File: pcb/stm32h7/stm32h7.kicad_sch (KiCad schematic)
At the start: 36 parts, among them SW2 SW_Push, SW3 SW_Push, U1 STM32H743VGTx, U11 TPS61169DCKR, U9 MT25QUxxxxxx1xW7, Y1 25MHz

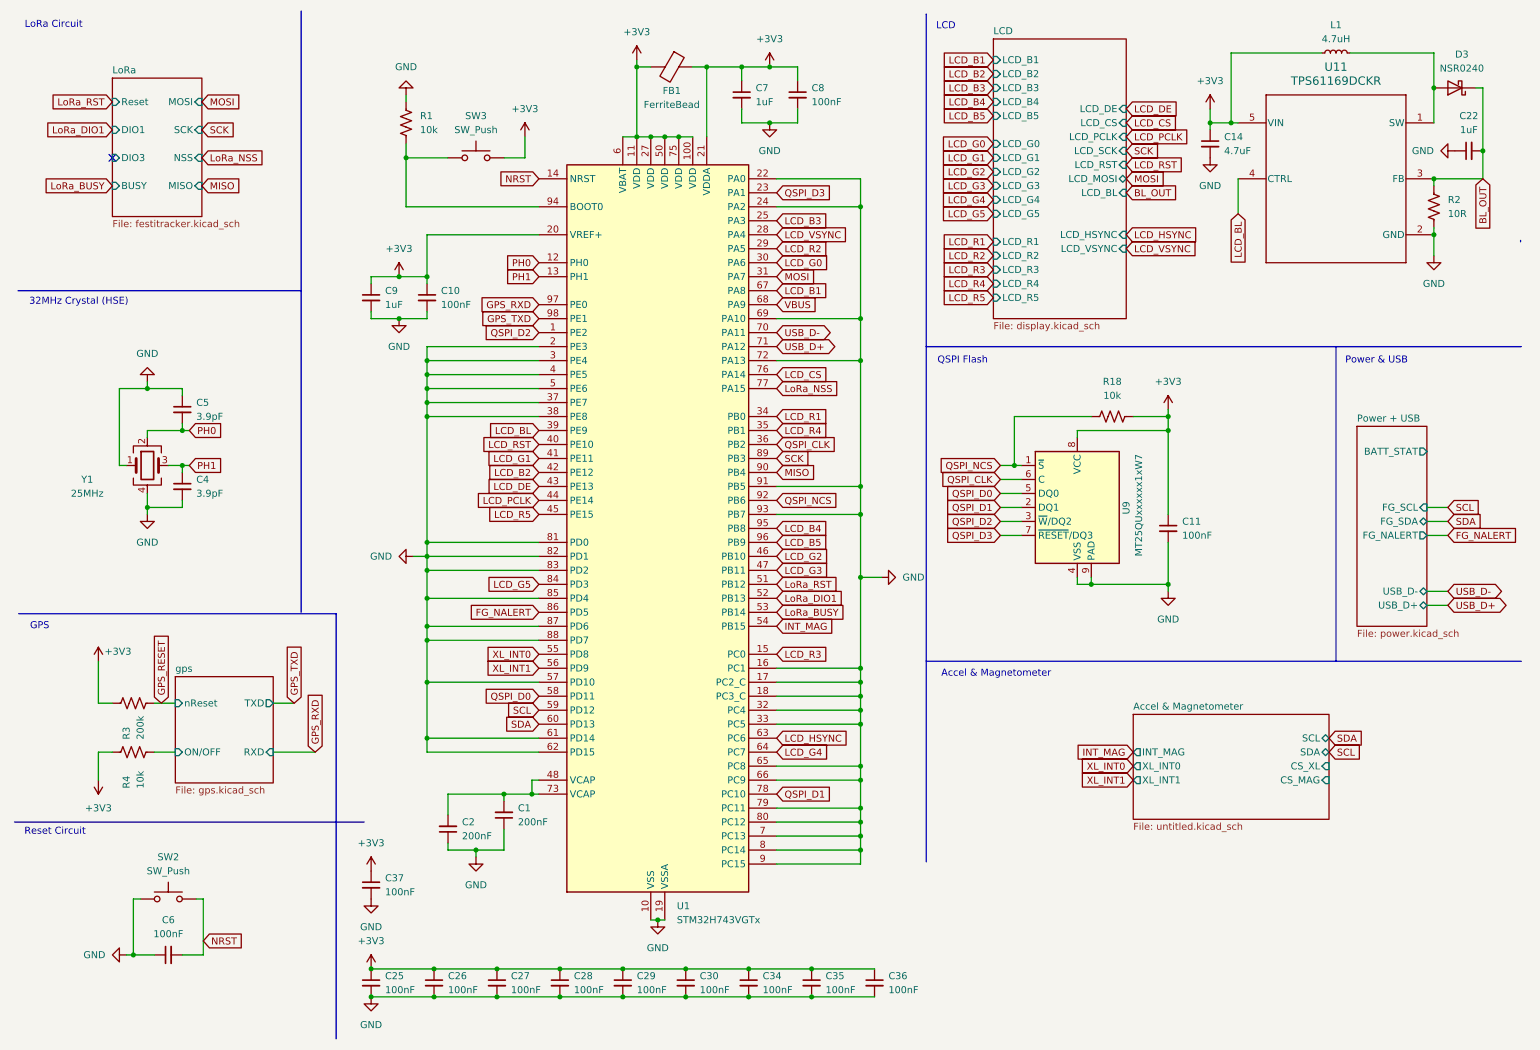
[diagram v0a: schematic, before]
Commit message: routing done
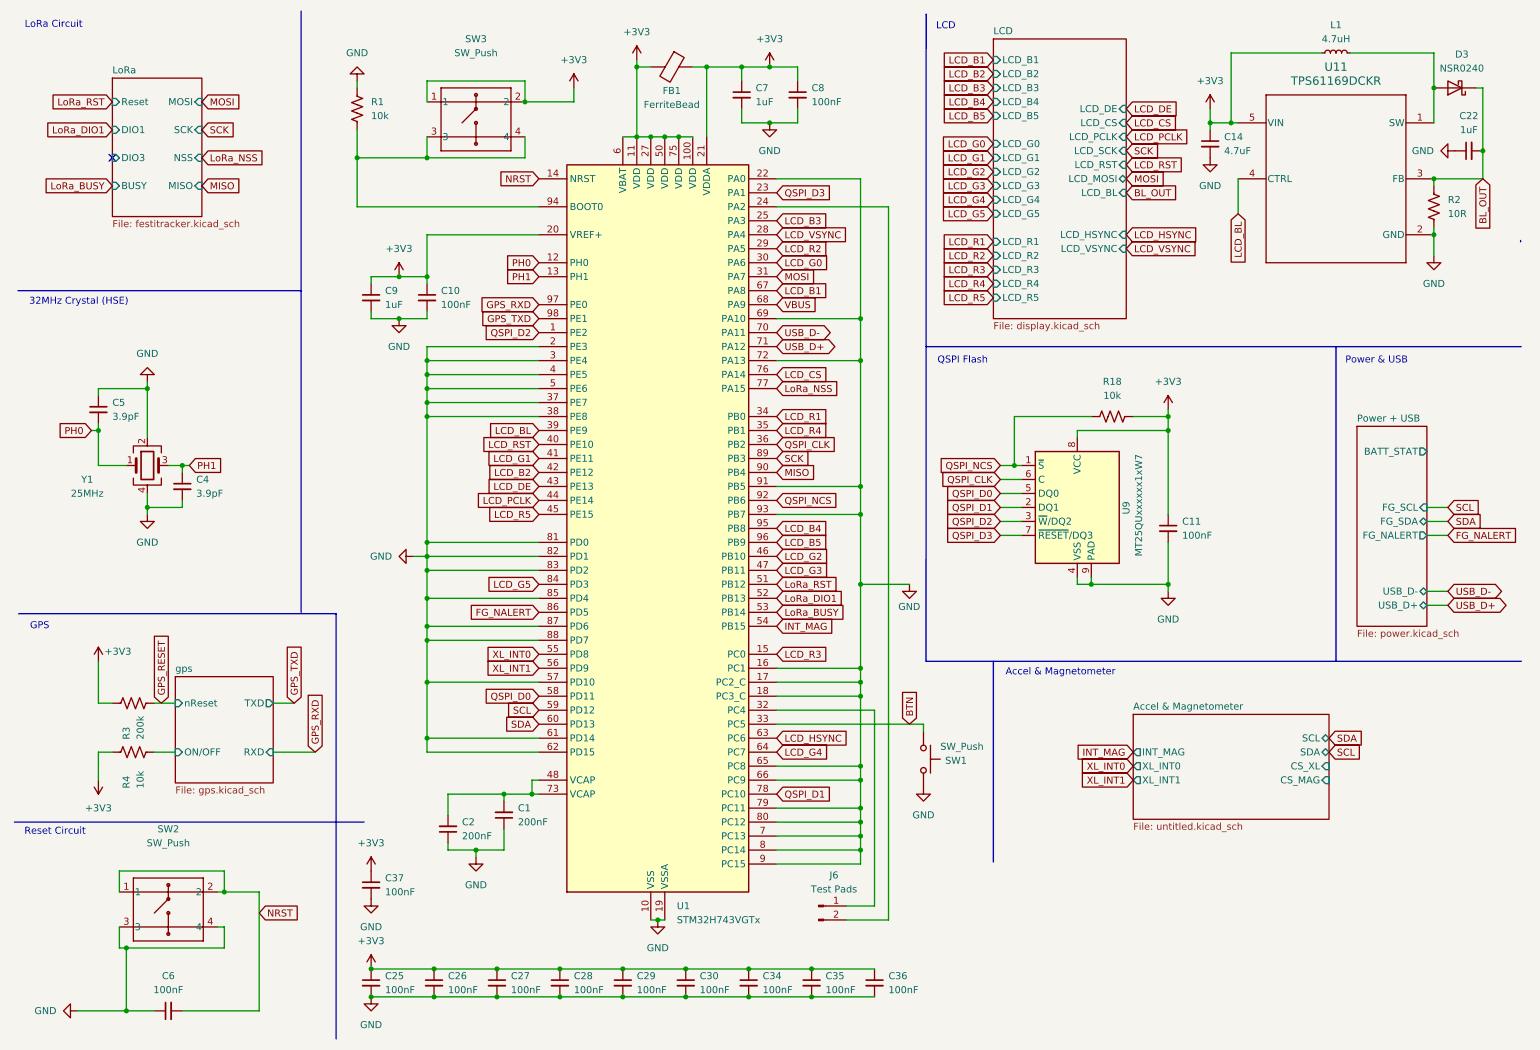
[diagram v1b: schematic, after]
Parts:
- removed SW3: SW_Push, custom_comps:SW4_PTS815 SJM 250 SMTR LFS_CNK, symbol Switch:SW_Push
- added J6: Test Pads, custom_comps:2 Wire Pads, symbol Connector:Conn_01x02_Pin
- added SW1: SW_Push, custom_comps:vert_button_6mm, symbol Switch:SW_Push
- added SW3: SW_Push, SW4_PTS815 SJM 250 SMTR LFS_CNK, symbol PTS815_SJM_250_SMTR_LFS:PTS815_SJM_250_SMTR_LFS
- C14, C22: footprint (none) -> Capacitor_SMD:C_0402_1005Metric
- R2: footprint (none) -> Resistor_SMD:R_0402_1005Metric
- SW2: footprint custom_comps:SW4_PTS815 SJM 250 SMTR LFS_CNK -> SW4_PTS815 SJM 250 SMTR LFS_CNK; symbol Switch:SW_Push -> PTS815_SJM_250_SMTR_LFS:PTS815_SJM_250_SMTR_LFS
- U11: footprint DCK0005A_N -> custom_comps:DCK0005A_N
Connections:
- net +3V3: now also SW3.1, SW3.2
- net GND: now also SW2.3, SW2.4, Y1.2, SW1.2; no longer SW2.1, U1.24 (PA2), U1.32 (PC4), U1.33 (PC5), Y1.1
- net NRST: now also SW2.1
- net PH0: now also Y1.1; no longer Y1.2
- net at R1.1, U1.94 (BOOT0): now also SW3.3, SW3.4
- new net: J6.1 (Pin_1), U1.32 (PC4)
- new net: J6.2 (Pin_2), U1.24 (PA2)
- new net BTN: SW1.1, U1.33 (PC5)
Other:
- moved on the sheet: C5, C6, R1
